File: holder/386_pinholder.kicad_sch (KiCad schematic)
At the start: 1 part

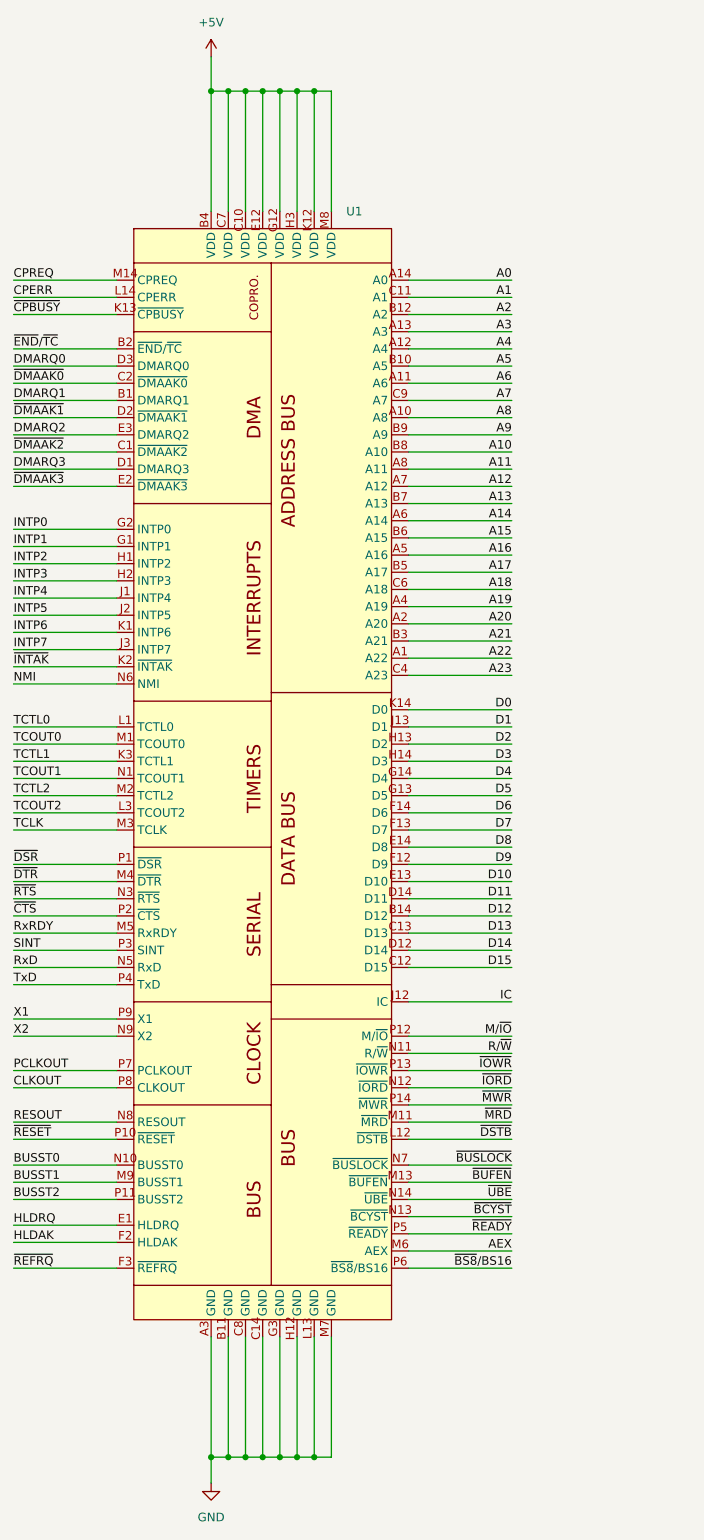
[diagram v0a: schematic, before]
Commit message: Update holder schematic and gerber
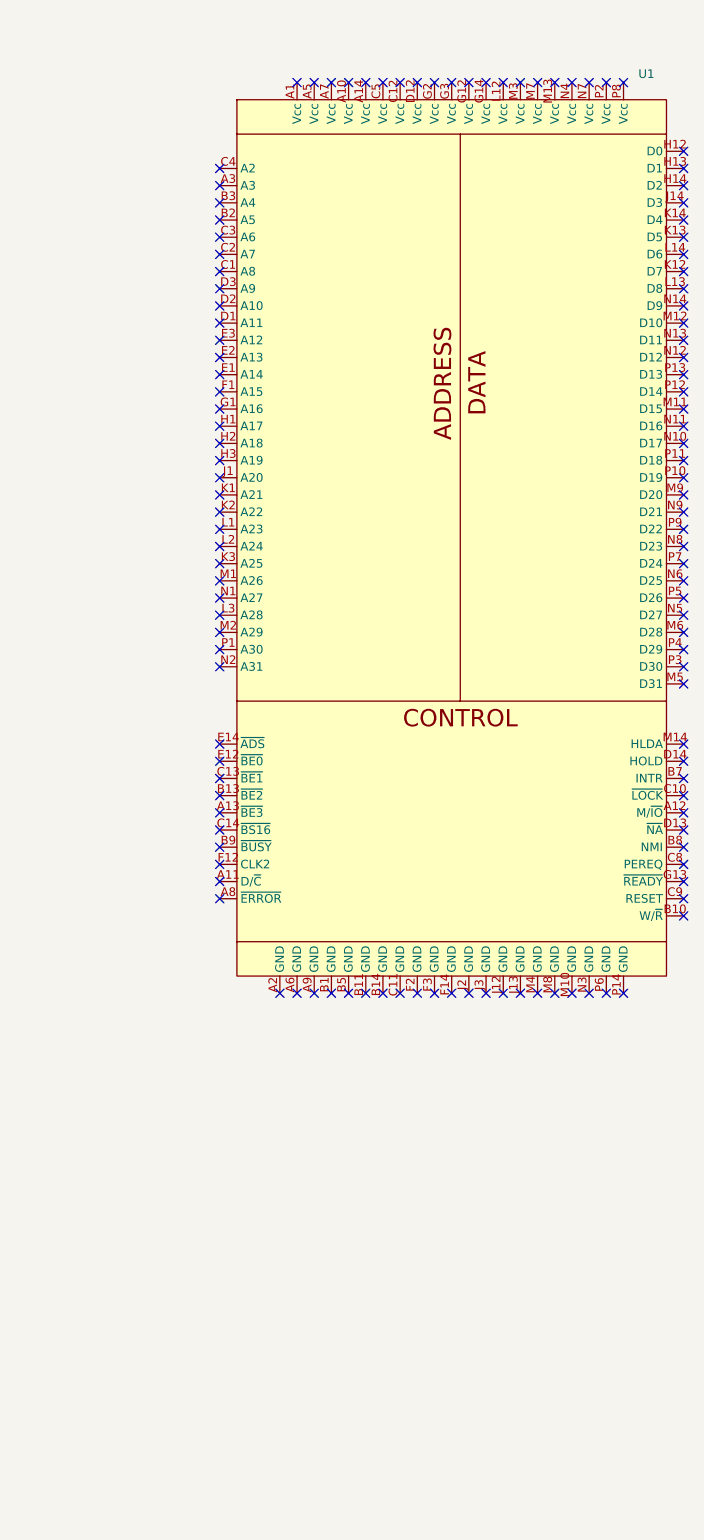
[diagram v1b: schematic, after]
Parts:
- removed U1: ~, Custom_PGA:PGA-132_holder, symbol V53:V53_PGA
- added U1: ~, Custom_PGA:PGA-132_holder, symbol AM386:AM386_PGA
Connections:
- no-connect marks 0 -> 124
